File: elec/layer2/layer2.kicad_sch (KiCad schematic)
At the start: 0 parts

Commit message: fix: l1 gnd
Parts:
- added J1: Conn_01x03, Pinheaders:PinHeader_1x03_P2.54mm_Vertical, symbol Connector_Generic:Conn_01x03
- added J2: XT30UPB-M, layer2-pcb-footprints:AMASS_XT30UPB-M, symbol layer2-pcb-symbols:XT30UPB-M
- added SW1: SW_SPDT_312, layer2-pcb-footprints:SS12D00G3, symbol Switch:SW_SPDT_312
- added TP1, TP2: TestPoint_2Pole, TestPoint:TestPoint_2Pads_Pitch2.54mm_Drill0.8mm, symbol Connector:TestPoint_2Pole
- added U1: TEENSY40, layer2-pcb-footprints:TEENSY40, symbol layer2-pcb-symbols:TEENSY40
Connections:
- new net +12V: J2.P
- new net +3V3: J1.1 (Pin_1), SW1.3 (A), TP2.1
- new net +5V: TP1.1
- new net Dribbler Data: J1.2 (Pin_2)
- new net GND: J1.3 (Pin_3), J2.N, SW1.2 (C), TP1.2, TP2.2, U1.G1
- new net Motors Enable: SW1.1 (B)
- no-connect marks 0 -> 13
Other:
- added sheet Motor 1 (motor.kicad_sch)
- added sheet Motor 2 (motor.kicad_sch)
- added sheet Motor 3 (motor.kicad_sch)
- added sheet Motor 4 (motor.kicad_sch)
- note added: "Dribbler"
- note added: "MCU"
- note added: "Motors"
- note added: "Motors Enable"
- note added: "Testpoints"
- company: (none) -> Chen-Xuan Ng
- title: (none) -> A PCB

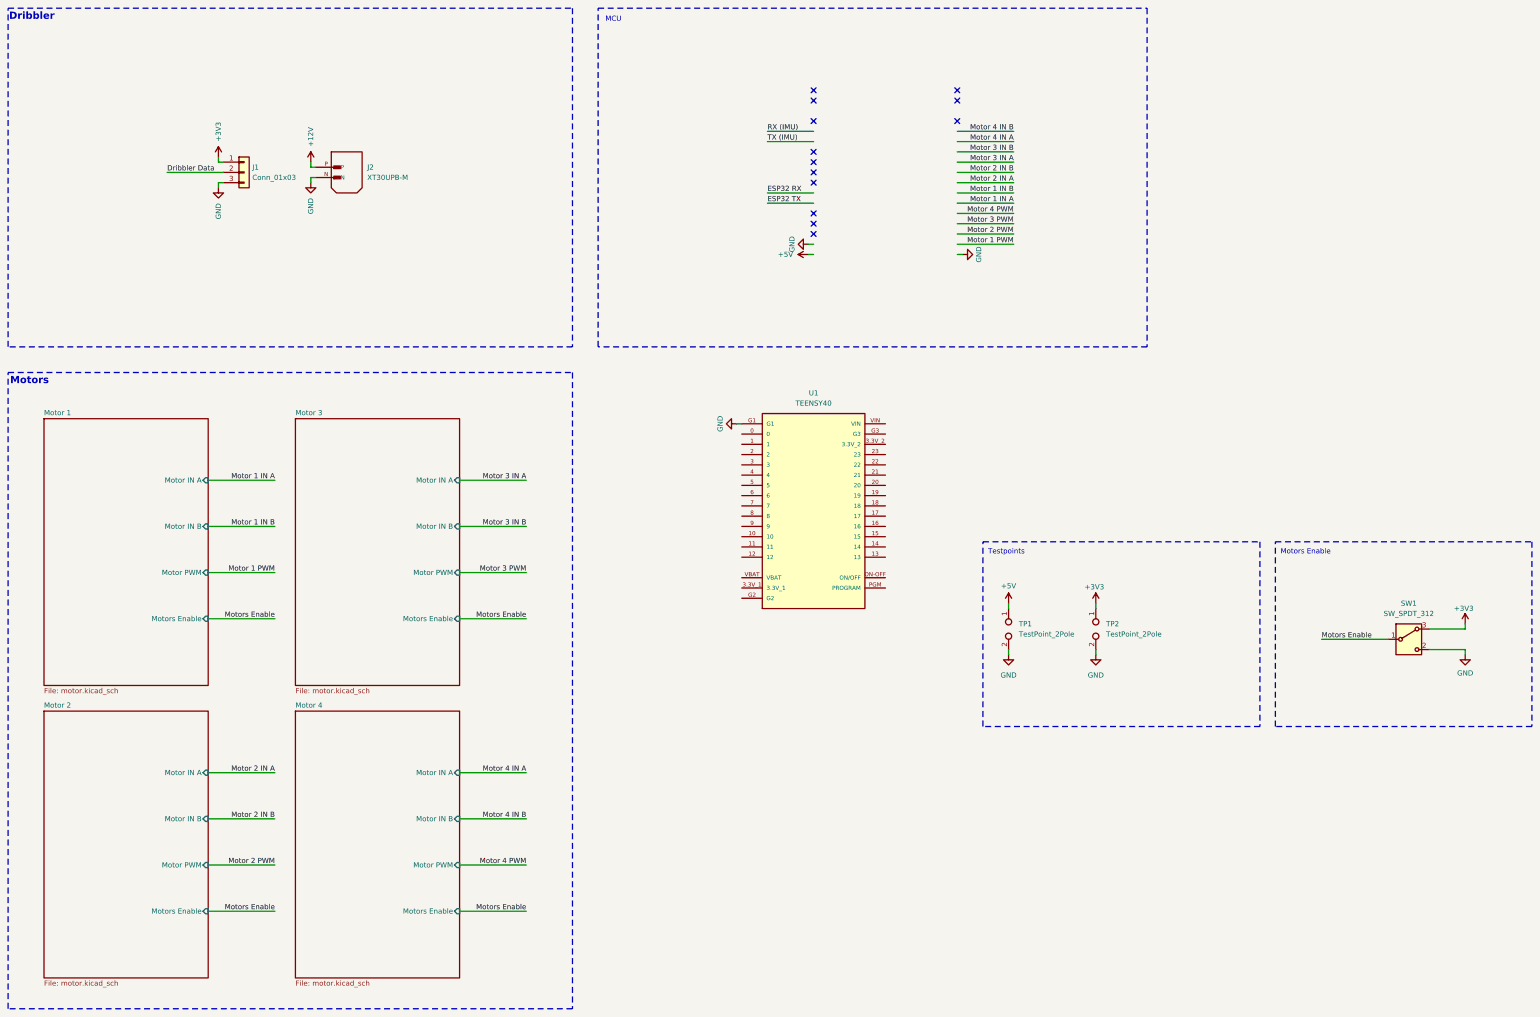
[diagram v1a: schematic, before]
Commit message: fix: l1; chore: l2 schematics
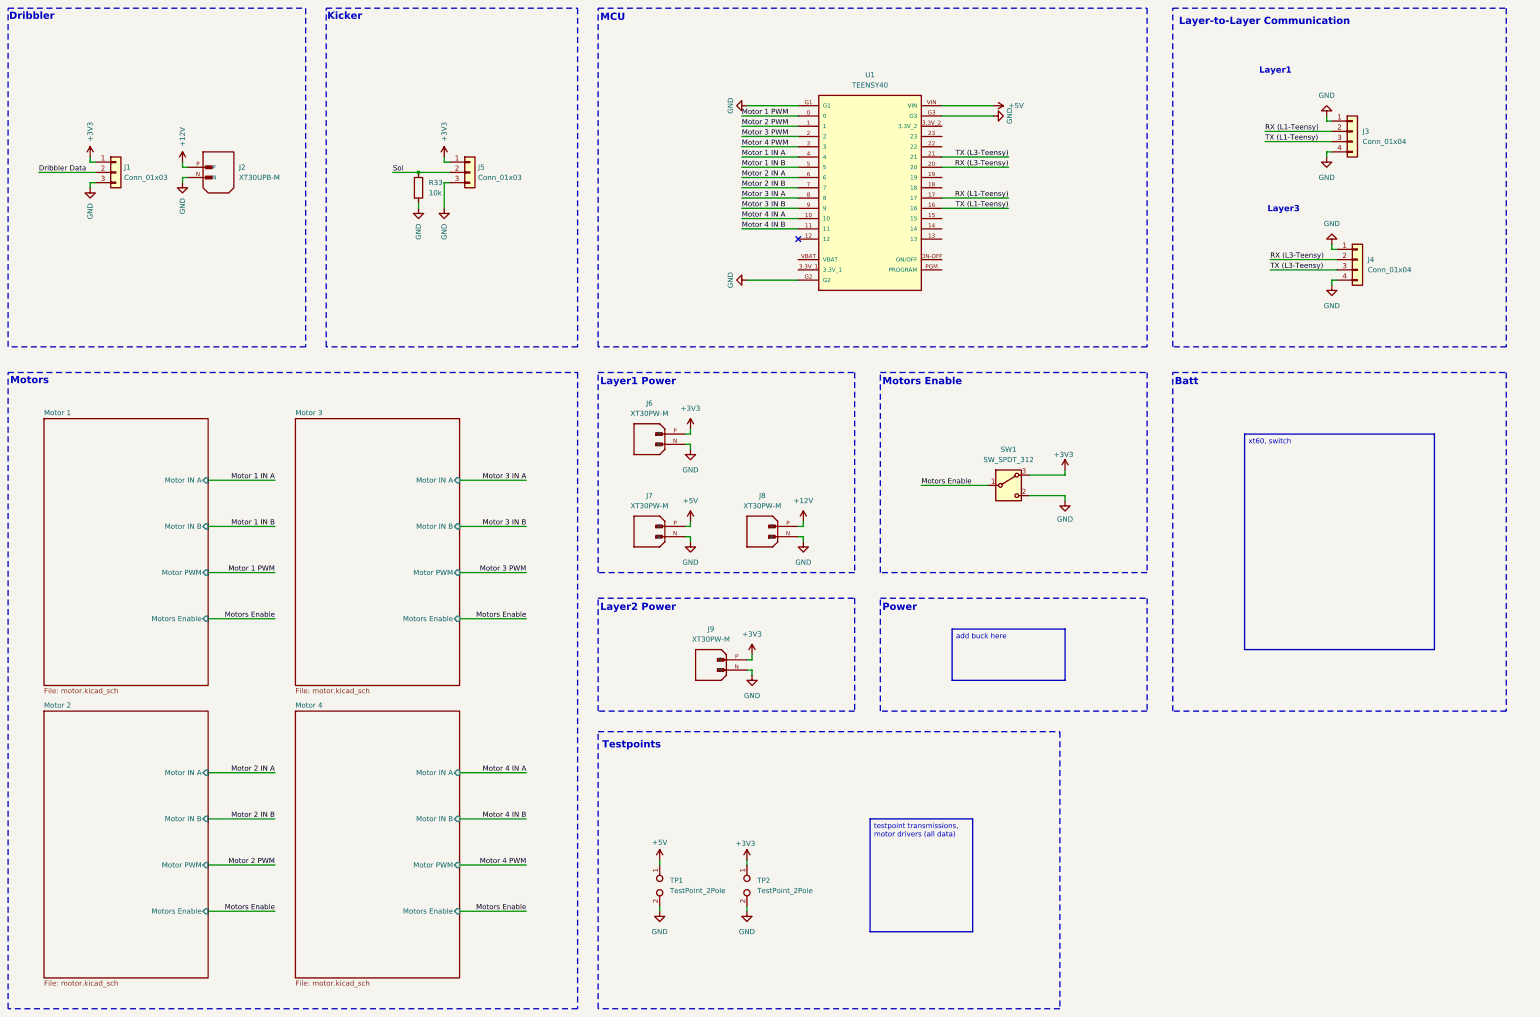
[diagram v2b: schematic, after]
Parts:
- added J3, J4: Conn_01x04, Connector_JST:JST_XH_B4B-XH-AM_1x04_P2.50mm_Vertical, symbol Connector_Generic:Conn_01x04
- added J5: Conn_01x03, Pinheaders:PinHeader_1x03_P2.54mm_Vertical, symbol Connector_Generic:Conn_01x03
- added J6, J7, J8, J9: XT30PW-M, layer1-pcb-footprints:AMASS_XT30PW-M, symbol layer1-pcb-symbols:XT30PW-M
- added R33: 10k, symbol Device:R
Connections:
- net +12V: now also J8.P
- net +3V3: now also J5.1 (Pin_1), J6.P, J9.P
- net +5V: now also U1.VIN, J7.P
- net GND: now also U1.G2, U1.G3, J3.1 (Pin_1), J3.4 (Pin_4), J4.1 (Pin_1), J4.4 (Pin_4), J5.3 (Pin_3), J6.N, J7.N, J8.N, J9.N, R33.2
- net Motor 1 IN A: now also U1.4
- net Motor 1 IN B: now also U1.5
- net Motor 1 PWM: now also U1.0
- net Motor 2 IN A: now also U1.6
- net Motor 2 IN B: now also U1.7
- net Motor 2 PWM: now also U1.1
- net Motor 3 IN A: now also U1.8
- net Motor 3 IN B: now also U1.9
- net Motor 3 PWM: now also U1.2
- net Motor 4 IN A: now also U1.10
- net Motor 4 IN B: now also U1.11
- net Motor 4 PWM: now also U1.3
- net TX (L1-Teensy): now reaches U1.16
- net TX (L1-Teensy): now also J3.3 (Pin_3)
- net RX (L1-Teensy): now reaches U1.17
- net RX (L1-Teensy): now also J3.2 (Pin_2)
- net RX (L3-Teensy): now reaches U1.20
- net RX (L3-Teensy): now also J4.2 (Pin_2)
- net TX (L3-Teensy): now reaches U1.21
- net TX (L3-Teensy): now also J4.3 (Pin_3)
- new net Sol: J5.2 (Pin_2), R33.1
- no-connect marks 13 -> 1
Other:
- note added: "Batt"
- note added: "Kicker"
- note added: "Layer-to-Layer Communication"
- note added: "Layer1"
- note added: "Layer1 Power"
- note added: "Layer2 Power"
- note added: "Layer3"
- note added: "Power"
- moved on the sheet: J1, J2, SW1, TP1, TP2, U1
